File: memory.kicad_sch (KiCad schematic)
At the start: 8 parts, among them U12 AS6C4008-55PCN, U26 SST39SF010, U7 AS6C4008-55PCN, U9 74LS245

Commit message: Upgraded speaker, esd protection, added dip sockets, adjusted routing
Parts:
- U12, U7: footprint Package_DIP:DIP-32_W15.24mm -> Package_DIP:DIP-32_W15.24mm_Socket
- U9: footprint Package_DIP:DIP-20_W7.62mm -> Package_DIP:DIP-20_W7.62mm_Socket
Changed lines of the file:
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@@
 			)
 		)
-		(property "Footprint" "Package_DIP:DIP-32_W15.24mm"
+		(property "Footprint" "Package_DIP:DIP-32_W15.24mm_Socket"
 			(at 154.94 119.38 0)
 			(hide yes)
@@
 		)
 		(property "Sim.Type" ""
+			(at 154.94 121.92 0)
+			(hide yes)
+			(show_name no)
+			(do_not_autoplace no)
+			(effects
+				(font
+					(size 1.27 1.27)
+				)
+			)
+		)
+		(property "Sim.Device" ""
 			(at 154.94 121.92 0)
 			(hide yes)
@@
 			)
 		)
+		(property "Sim.Device" ""
+			(at 257.81 27.94 0)
+			(hide yes)
+			(show_name no)
+			(do_not_autoplace no)
+			(effects
+				(font
+					(size 1.27 1.27)
+				)
+			)
+		)
 		(pin "2"
 		)
@@
 			)
 		)
+		(property "Sim.Device" ""
+			(at 229.87 27.94 0)
+			(hide yes)
+			(show_name no)
+			(do_not_autoplace no)
+			(effects
+				(font
+					(size 1.27 1.27)
+				)
+			)
+		)
 		(pin "2"
 		)
@@
 			)
 		)
+		(property "Sim.Device" ""
+			(at 271.78 27.94 0)
+			(hide yes)
+			(show_name no)
+			(do_not_autoplace no)
+			(effects
+				(font
+					(size 1.27 1.27)
+				)
+			)
+		)
 		(pin "2"
 		)
@@
 			)
 		)
+		(property "Sim.Device" ""
+			(at 243.84 27.94 0)
+			(hide yes)
+			(show_name no)
+			(do_not_autoplace no)
+			(effects
+				(font
+					(size 1.27 1.27)
+				)
+			)
+		)
 		(pin "2"
 		)
@@
 			)
 		)
-		(property "Footprint" "Package_DIP:DIP-32_W15.24mm"
+		(property "Footprint" "Package_DIP:DIP-32_W15.24mm_Socket"
 			(at 154.94 198.12 0)
 			(hide yes)
@@
 		)
 		(property "Sim.Type" ""
+			(at 154.94 200.66 0)
+			(hide yes)
+			(show_name no)
+			(do_not_autoplace no)
+			(effects
+				(font
+					(size 1.27 1.27)
+				)
+			)
+		)
+		(property "Sim.Device" ""
 			(at 154.94 200.66 0)
 			(hide yes)
@@
 			)
 		)
+		(property "Sim.Device" ""
+			(at 154.94 304.8 0)
+			(hide yes)
+			(show_name no)
+			(do_not_autoplace no)
+			(effects
+				(font
+					(size 1.27 1.27)
+				)
+			)
+		)
 		(pin "27"
 		)
@@
 			)
 		)
-		(property "Footprint" "Package_DIP:DIP-20_W7.62mm"
+		(property "Footprint" "Package_DIP:DIP-20_W7.62mm_Socket"
 			(at 154.94 57.15 0)
 			(hide yes)
@@
 			(at 154.94 57.15 0)
 			(hide yes)
+			(show_name no)
+			(do_not_autoplace no)
+			(effects
+				(font
+					(size 1.27 1.27)
+				)
+			)
+		)
+		(property "Sim.Device" ""
+			(at 154.94 57.15 0)
+			(hide yes)

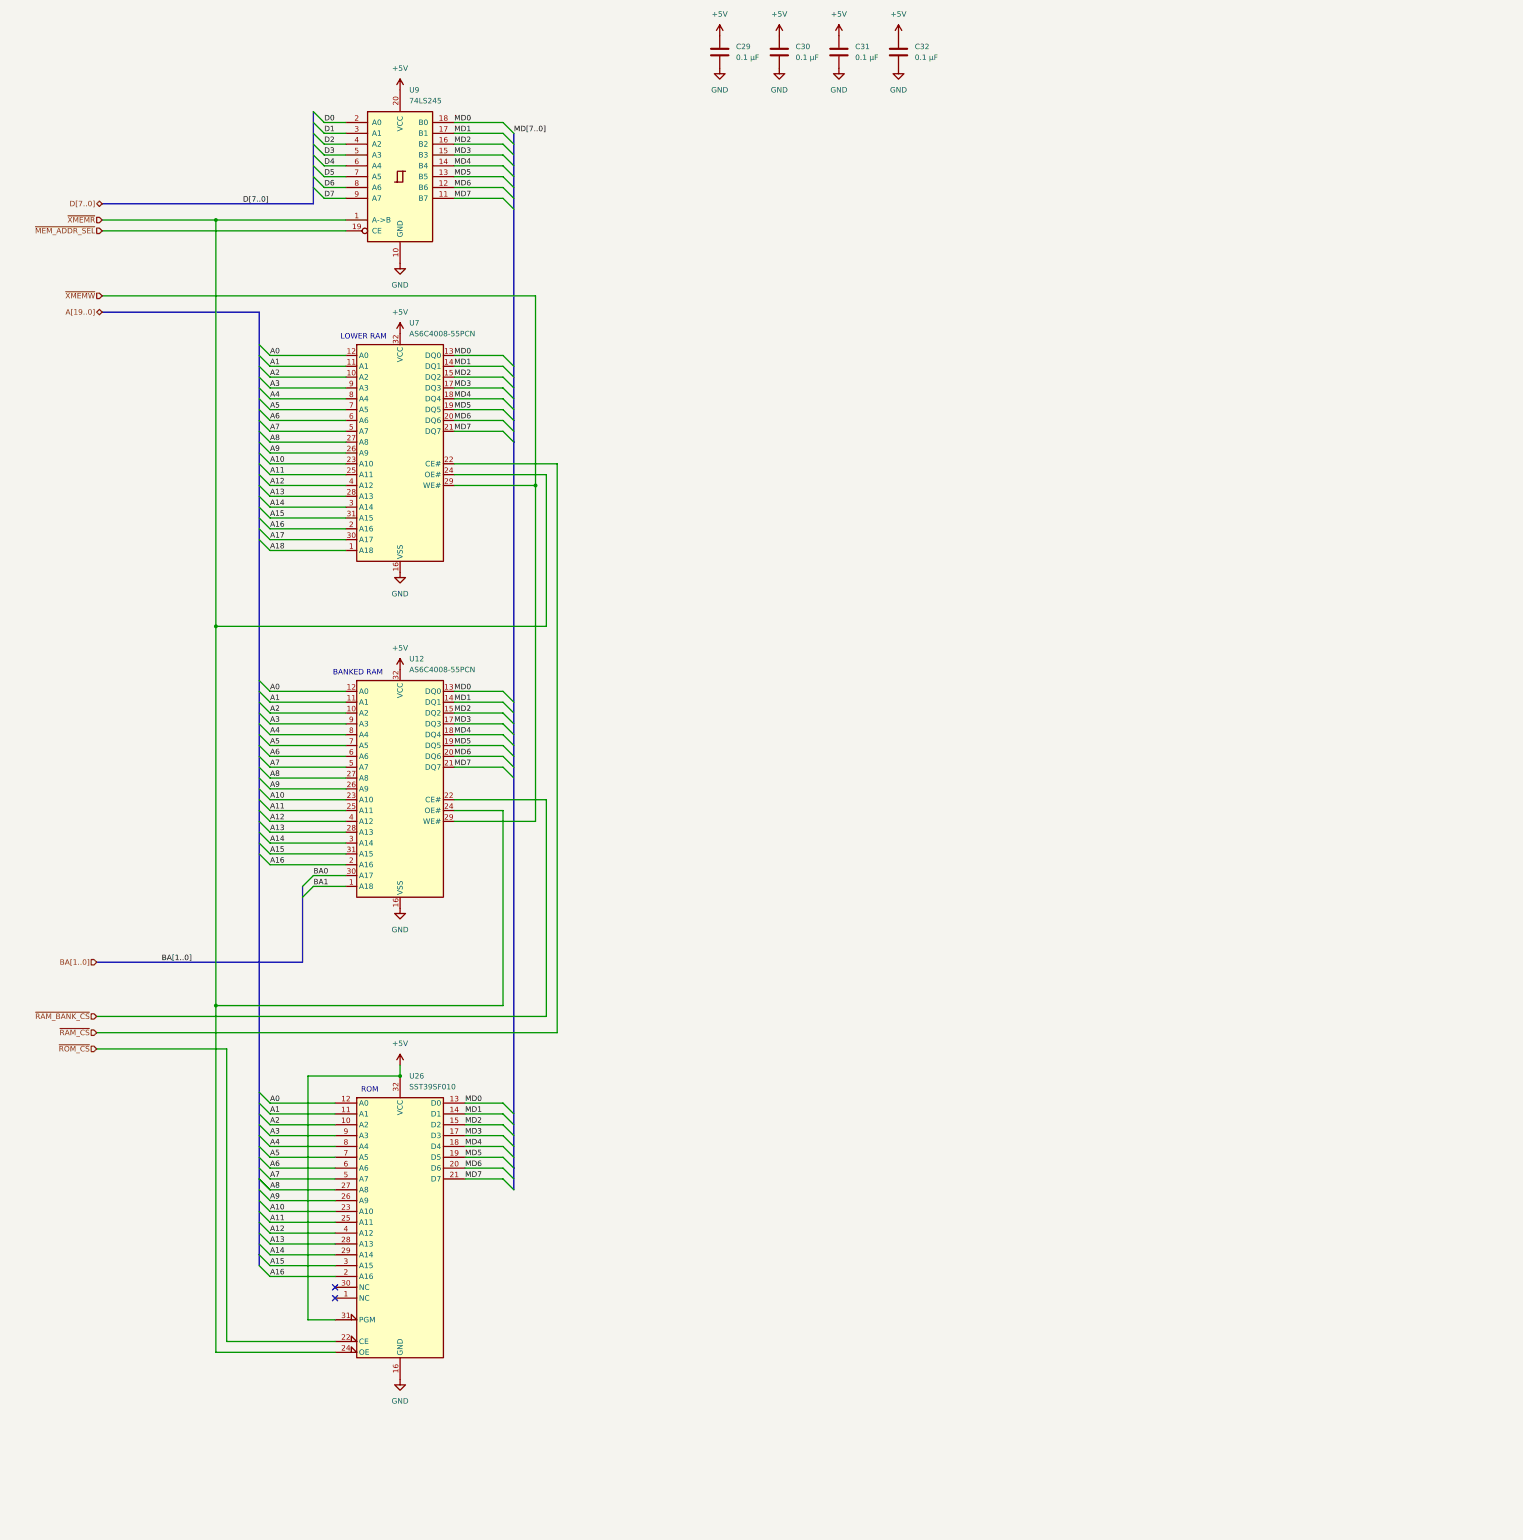
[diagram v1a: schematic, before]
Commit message: final final review
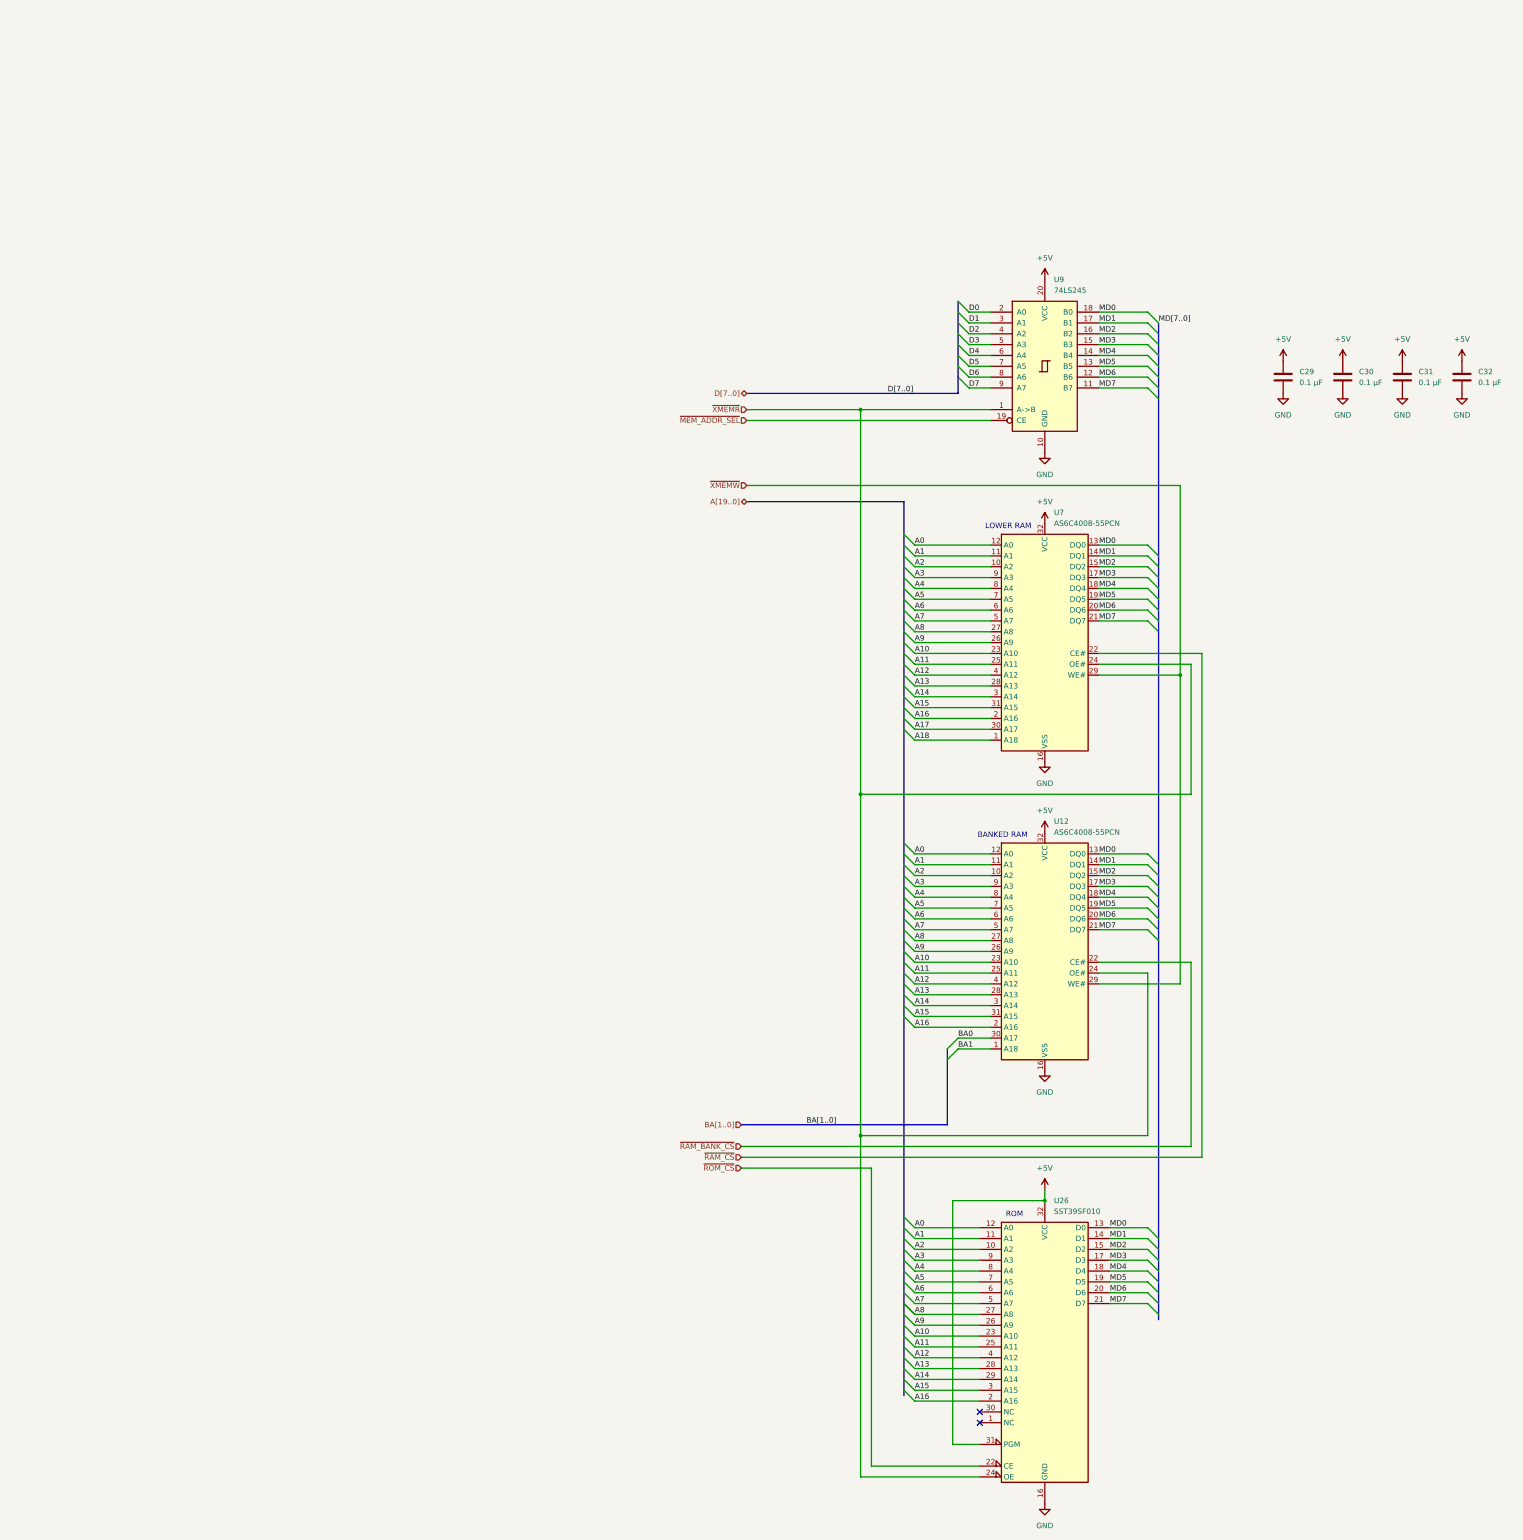
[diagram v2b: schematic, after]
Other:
- moved on the sheet: C29, C30, C31, C32, U12, U26, U7, U9
